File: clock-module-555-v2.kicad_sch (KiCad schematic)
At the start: 37 parts, among them J1 Conn_01x03_Pin, J2 Conn_01x03_Socket, SW1 MODE, SW2 PULSE, U1 NE555P, U2 74HC112, U3 NE555P, U4 74HC00, U5 NE555P

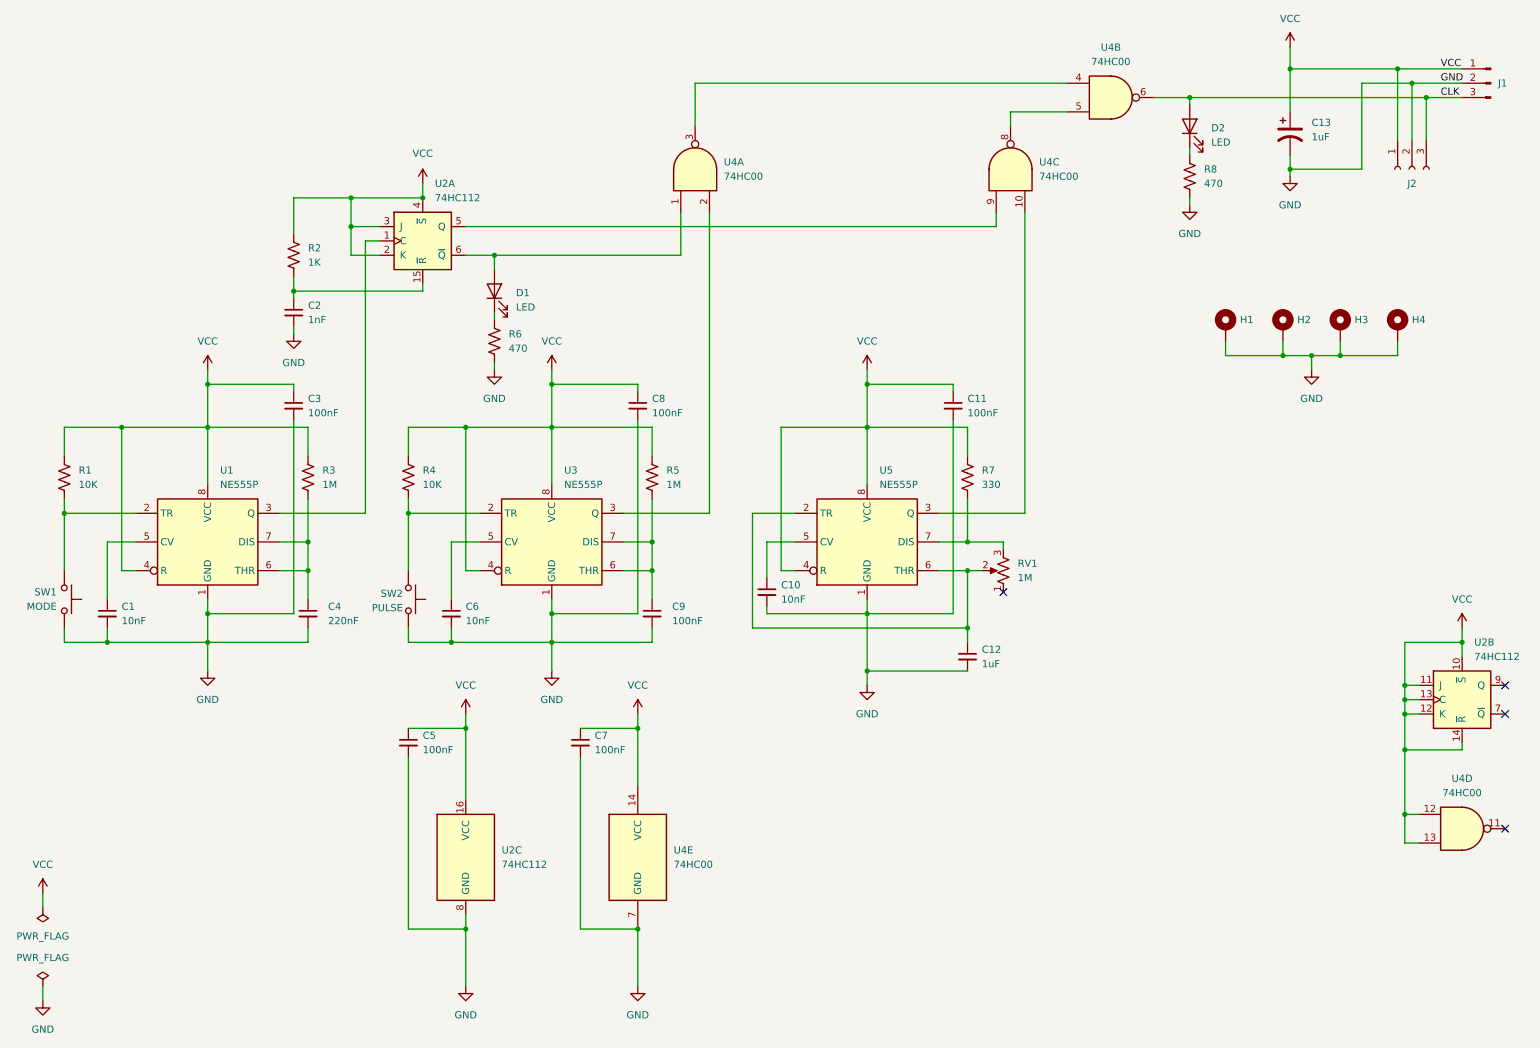
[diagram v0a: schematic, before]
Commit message: marked as rev 2
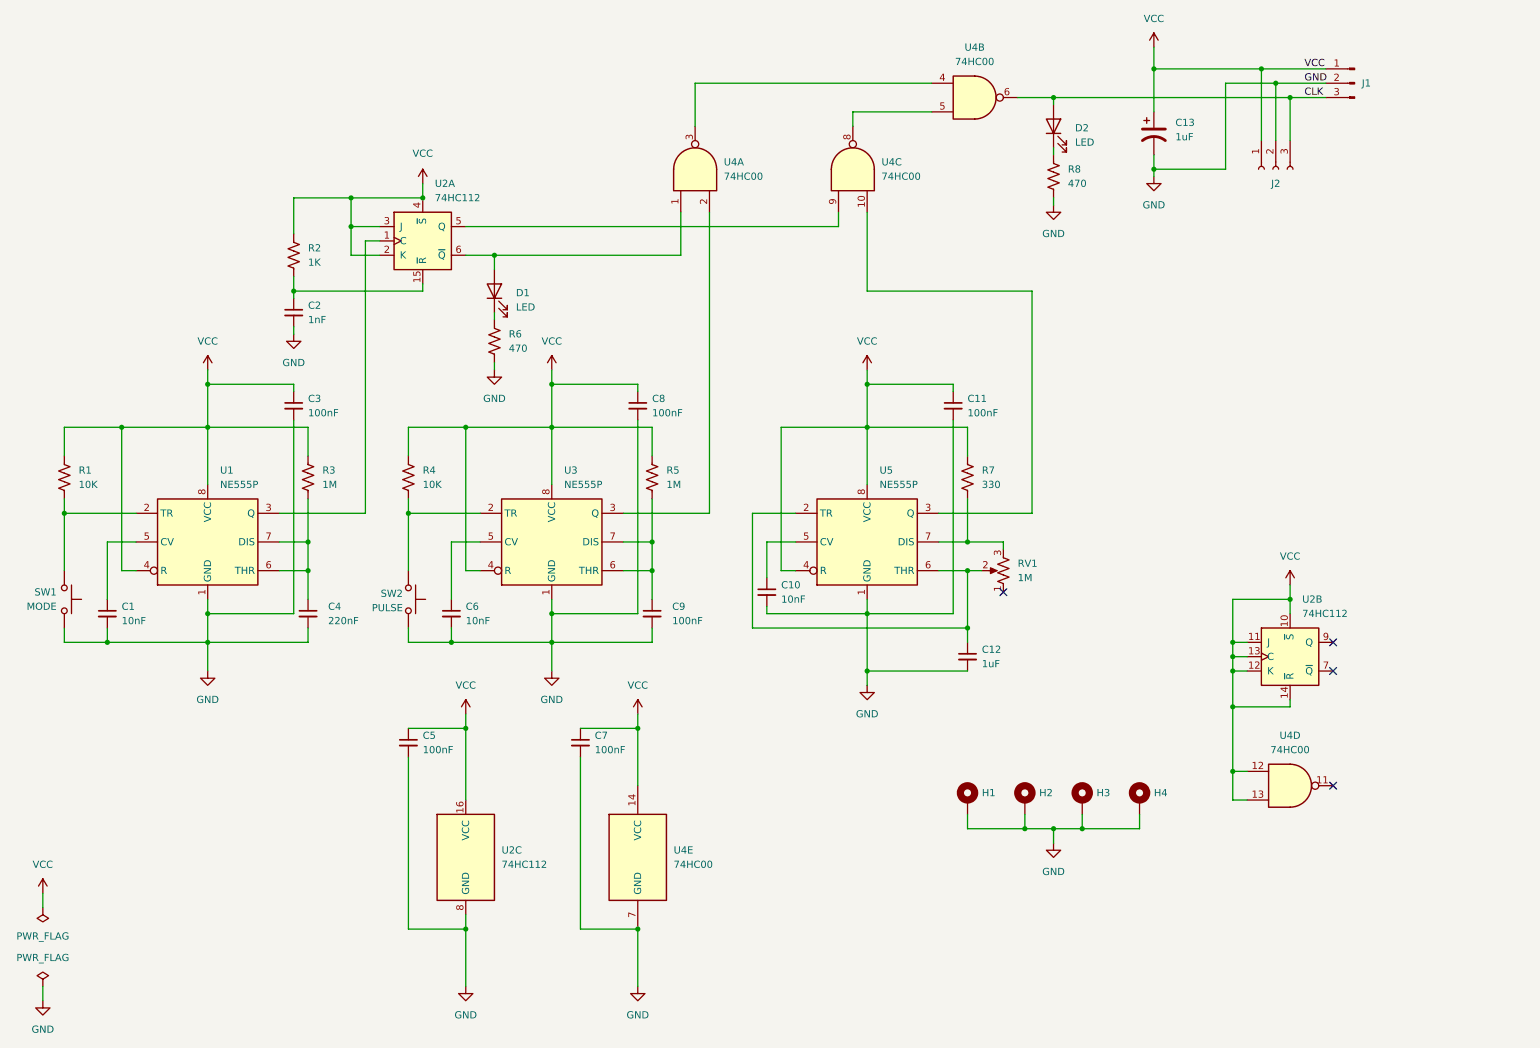
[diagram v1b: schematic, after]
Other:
- moved on the sheet: C13, D2, H1, H2, H3, H4, J1, J2, R8, U2B, U4B, U4C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
